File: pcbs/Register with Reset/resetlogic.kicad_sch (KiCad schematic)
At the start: 12 parts, among them U401 74HC08, U402 74HC14

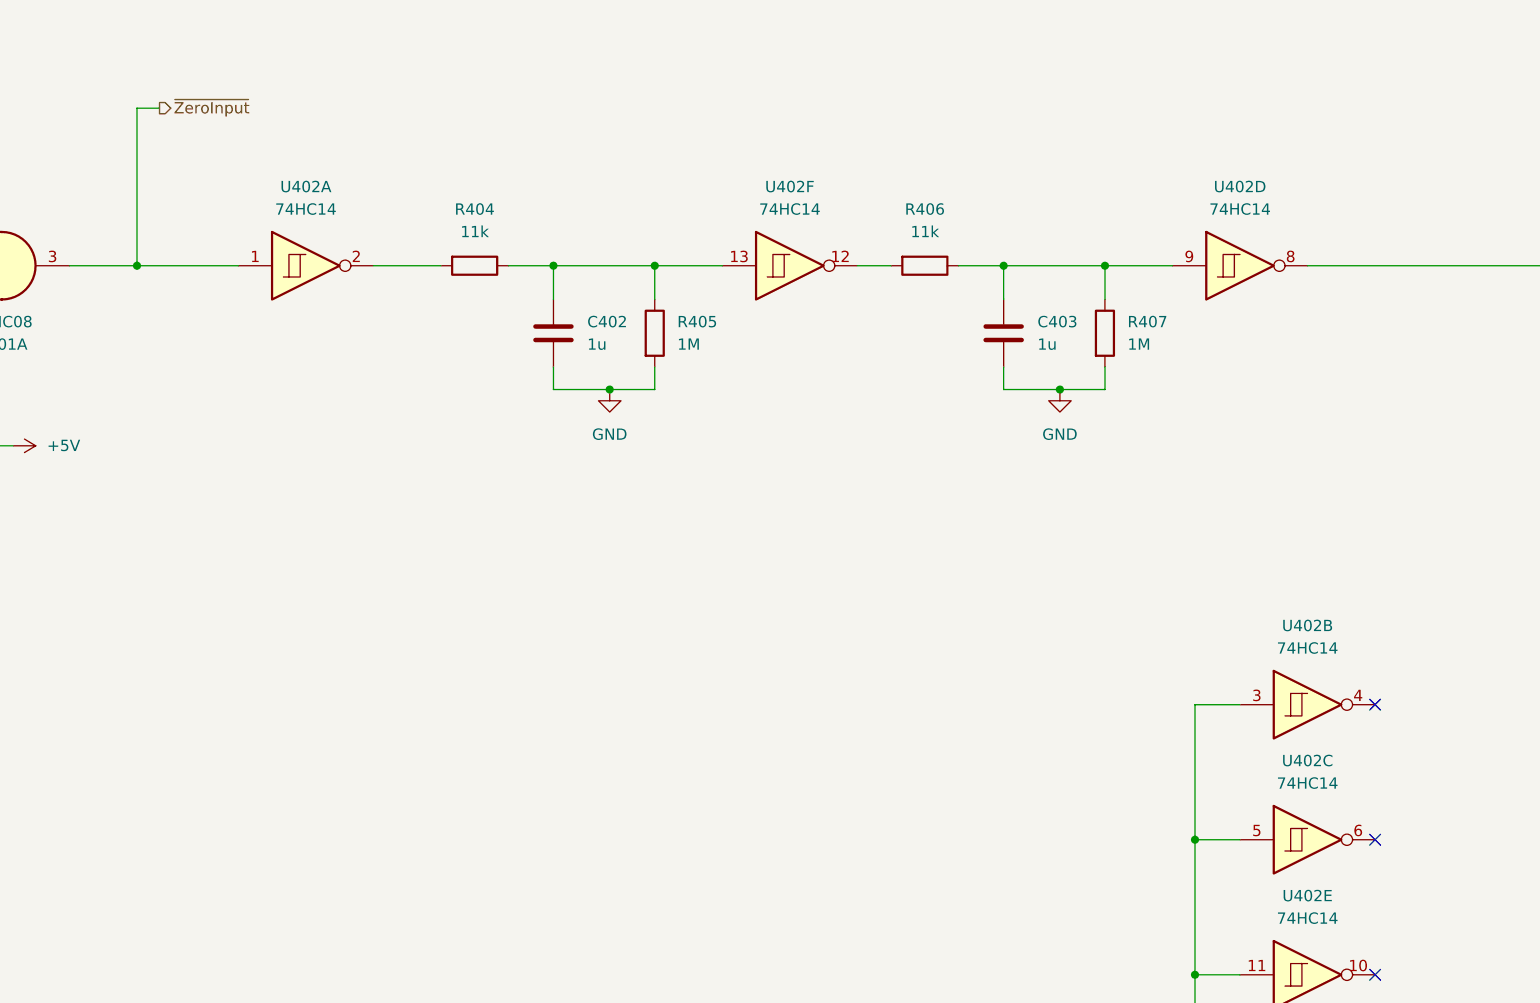
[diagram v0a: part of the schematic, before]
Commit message: Fix the reset logic....
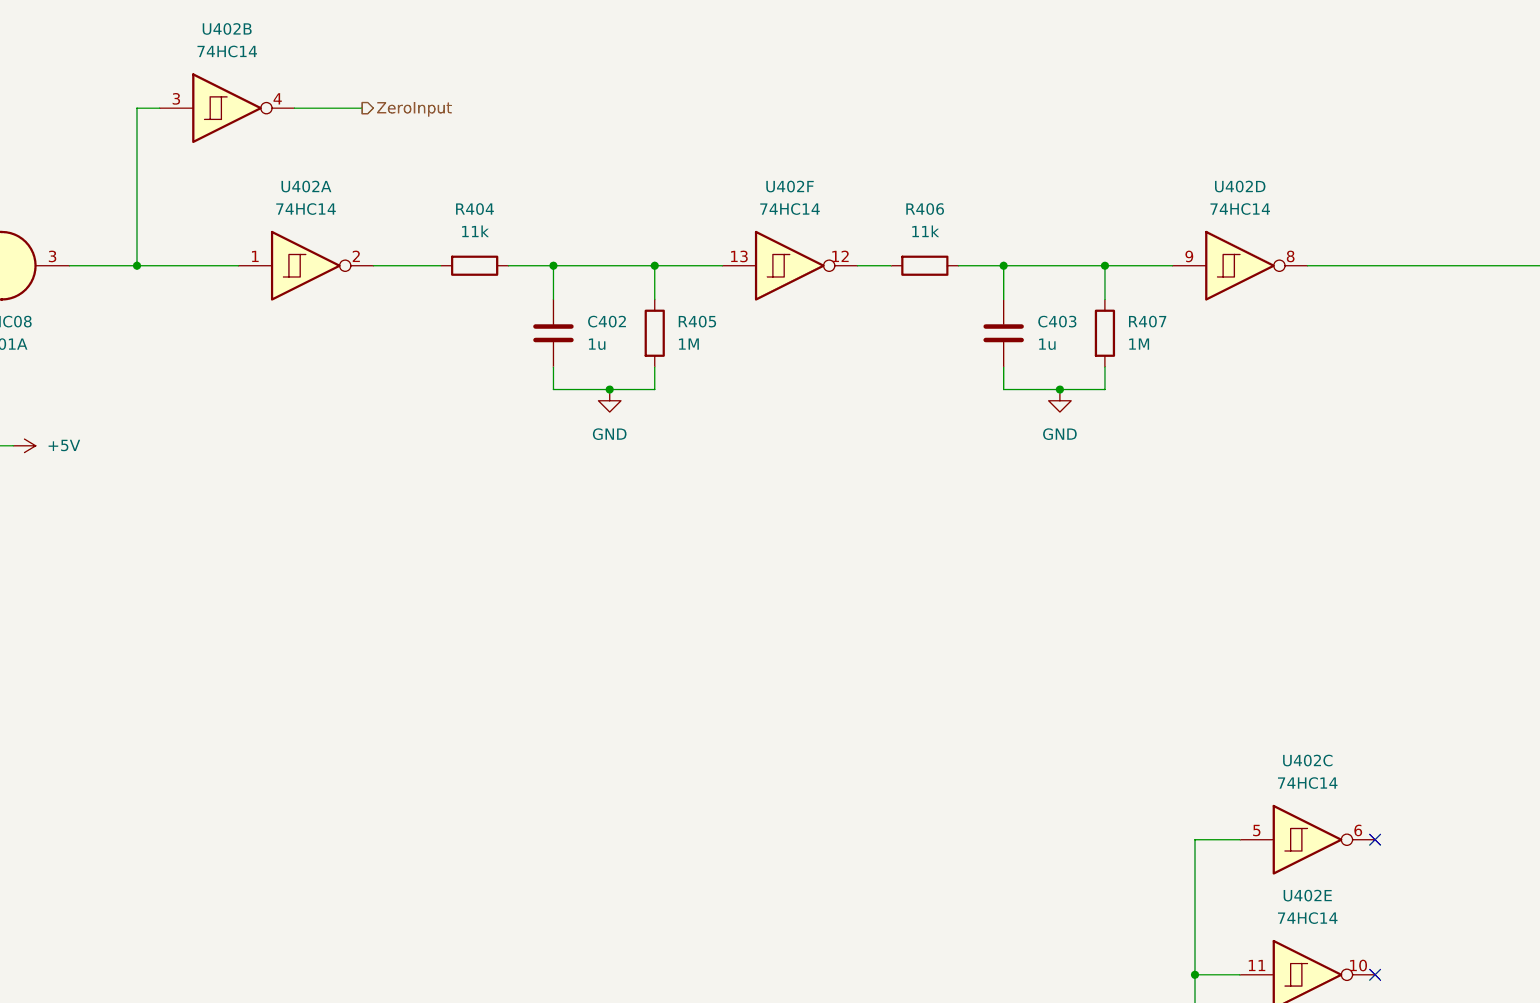
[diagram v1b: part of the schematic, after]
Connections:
- net GND: no longer U402.3
- net ZeroInput: now reaches U402.4
- net ~{ZeroInput}: no longer names the net of U401.3, U402.1
- net ~{ZeroInput}: now also U402.3
- no-connect marks 6 -> 5
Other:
- moved on the sheet: U402B
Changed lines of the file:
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@@
-	)
-	(junction
-		(at 205.74 120.65)
-		(diameter 0)
-		(color 0 0 0 0)
 	)
 	(junction
@@
 		(at 39.37 162.56)
 	)
-	(no_connect
-		(at 226.06 105.41)
-	)
 	(wire
 		(pts
@@
 	(wire
 		(pts
-			(xy 205.74 120.65) (xy 205.74 105.41)
-		)
-		(stroke
-			(width 0)
-			(type default)
-		)
-	)
-	(wire
-		(pts
 			(xy 25.4 53.34) (xy 35.56 53.34)
 		)
@@
 	(wire
 		(pts
+			(xy 104.14 38.1) (xy 111.76 38.1)
+		)
+		(stroke
+			(width 0)
+			(type default)
+		)
+	)
+	(wire
+		(pts
 			(xy 144.78 55.88) (xy 152.4 55.88)
 		)
@@
 		(pts
 			(xy 21.59 144.78) (xy 24.13 144.78)
-		)
-		(stroke
-			(width 0)
-			(type default)
-		)
-	)
-	(wire
-		(pts
-			(xy 205.74 105.41) (xy 210.82 105.41)
 		)
 		(stroke
@@
 		)
 	)
-	(hierarchical_label "~{ZeroInput}"
+	(hierarchical_label "ZeroInput"
 		(shape output)
-		(at 88.9 38.1 0)
+		(at 111.76 38.1 0)
 		(fields_autoplaced yes)
 		(effects
@@
 	(symbol
 		(lib_id "74xx:74HC14")
-		(at 218.44 105.41 0)
+		(at 96.52 38.1 0)
 		(unit 2)
 		(exclude_from_sim no)
@@
 		(fields_autoplaced yes)
 		(property "Reference" "U402"
-			(at 218.44 96.52 0)
+			(at 96.52 29.21 0)
 			(effects
 				(font
@@
 		)
 		(property "Value" "74HC14"
-			(at 218.44 99.06 0)
+			(at 96.52 31.75 0)
 			(effects
 				(font
@@
 		)
 		(property "Footprint" "Package_SO:SOIC-14_3.9x8.7mm_P1.27mm"
-			(at 218.44 105.41 0)
+			(at 96.52 38.1 0)
 			(effects
 				(font
@@
 		)
 		(property "Datasheet" "https://wmsc.lcsc.com/wmsc/upload/file/pdf/v2/lcsc/1811141851_Nexperia-74HC14D-653_C5605.pdf"
-			(at 218.44 105.41 0)
+			(at 96.52 38.1 0)
 			(effects
 				(font
@@
 		)
 		(property "Description" "Hex inverter schmitt trigger"
-			(at 218.44 105.41 0)
+			(at 96.52 38.1 0)
 			(effects
 				(font
@@
 		)
 		(property "LCSC" "C5605"
-			(at 218.44 105.41 0)
-			(effects
-				(font
+			(at 96.52 38.1 0)
+			(effects
+				(font
